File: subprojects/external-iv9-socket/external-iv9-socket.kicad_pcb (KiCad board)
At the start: 2 copper layers, 20.1 x 15.1 mm, 3 parts, among them J1 PINHD_1x5_Male, J3 PINHD_1x4_Male

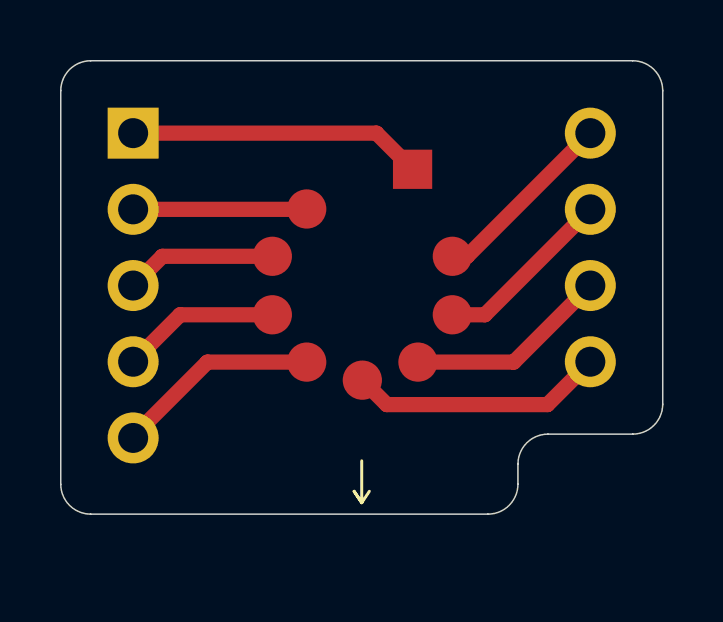
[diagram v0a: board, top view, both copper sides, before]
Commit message: Veľké pokroky pri navrhu DPS.
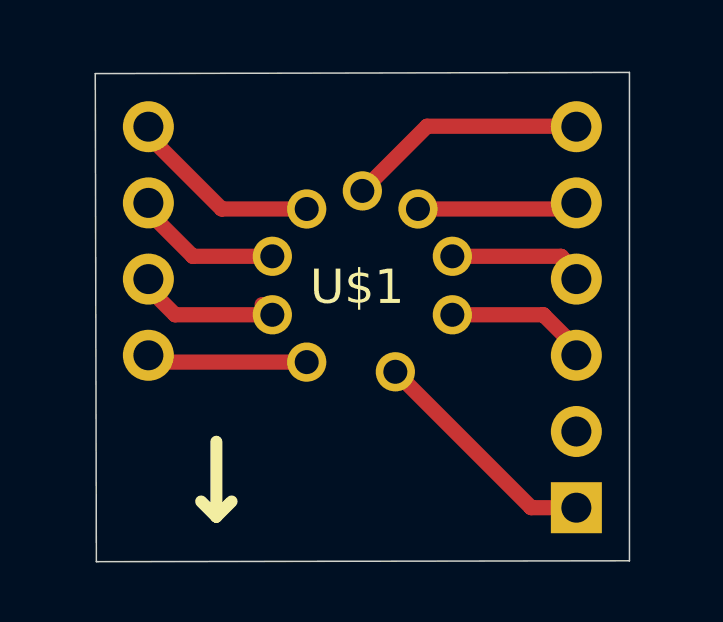
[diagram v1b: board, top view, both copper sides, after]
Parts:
- J1: value PINHD_1x5_Male -> PINHD_1x6_Male; footprint Connector_PinHeader_2.54mm:PinHeader_1x05_P2.54mm_Vertical -> Connector_PinHeader_2.54mm:PinHeader_1x06_P2.54mm_Vertical
- U$1: footprint VacuumTubes:IV-9 -> VacuumTubes:IV-9-Common-Separated
- moved J1 19.3 mm to (108.5, 81.7), turned to 0 degrees
- moved J3 14.7 mm to (94.2, 69.0)
- turned U$1 to 0 degrees
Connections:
- J1 pad 2: Net-(J1-Pad2) -> unconnected-(J1-Pad2)
- U$1 pad 2: Net-(J3-Pad1) -> Net-(J1-Pad3)
- U$1 pad 3: Net-(J3-Pad2) -> Net-(J1-Pad4)
- U$1 pad 4: Net-(J3-Pad3) -> Net-(J1-Pad5)
- U$1 pad 5: Net-(J3-Pad4) -> Net-(J1-Pad6)
- U$1 pad 6: Net-(J1-Pad5) -> Net-(J3-Pad1)
- U$1 pad 7: Net-(J1-Pad4) -> Net-(J3-Pad2)
- U$1 pad 8: Net-(J1-Pad3) -> Net-(J3-Pad3)
- U$1 pad 9: Net-(J1-Pad2) -> Net-(J3-Pad4)
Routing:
- net Net-(J1-Pad6): track 0.00 -> 8.26 mm
- net Net-(J1-Pad2): track 5.79 -> 0.00 mm
- net Net-(J3-Pad4): track 8.53 -> 5.61 mm
- net Net-(J1-Pad1): track 9.81 -> 7.91 mm
- net Net-(J3-Pad3): track 6.80 -> 5.34 mm
- net Net-(J3-Pad2): track 6.06 -> 5.10 mm
- net Net-(J1-Pad5): track 6.86 -> 5.91 mm
- net Net-(J1-Pad4): track 5.29 -> 4.68 mm
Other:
- board size 20.1 x 15.1 mm -> 17.8 x 16.3 mm
